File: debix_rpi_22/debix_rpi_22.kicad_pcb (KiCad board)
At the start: 2 copper layers, 71 x 12.5 mm, 2 parts, among them J1 Conn_01x24, J3 RPi 22 Pin MIPI CSI-2

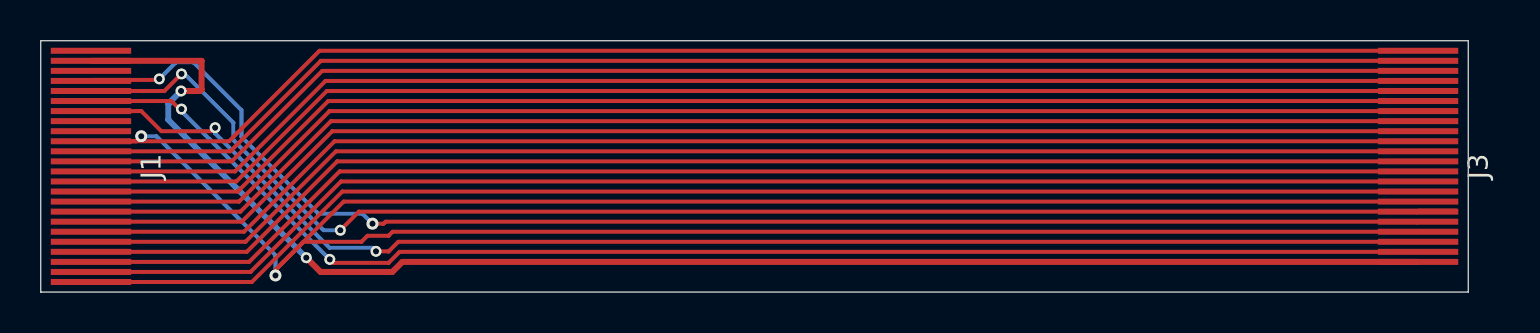
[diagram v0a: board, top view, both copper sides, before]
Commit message: ROUNDED.
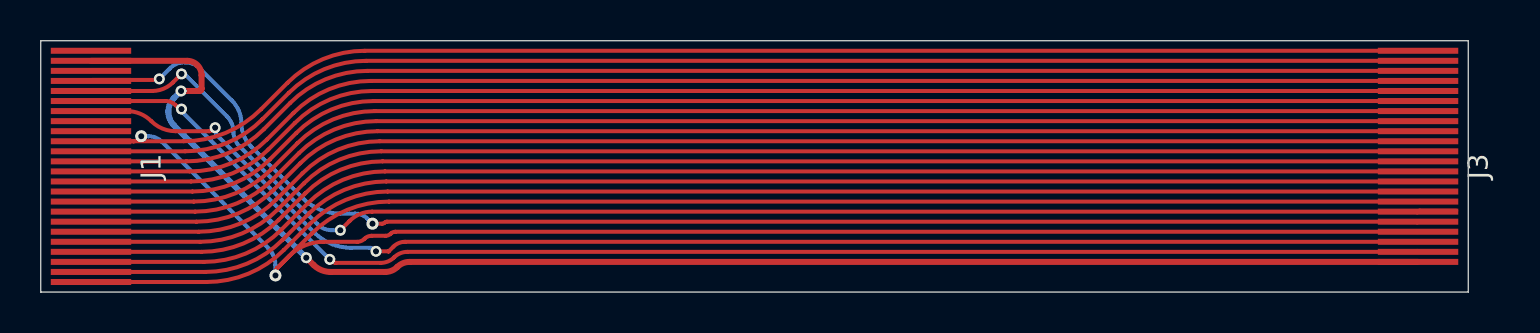
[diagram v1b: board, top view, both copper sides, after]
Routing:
- net GND: track 466.2 -> 463.2 mm
- net +3V3: track 75.2 -> 74.6 mm
- net /csi_d3_P: track 67.9 -> 67.3 mm
- net /csi_d3_N: track 67.9 -> 67.3 mm
- net /csi_d2_P: track 67.9 -> 67.3 mm
- net /csi_clk_N: track 67.9 -> 67.3 mm
- net /csi_d2_N: track 67.9 -> 67.3 mm
- net /csi_d1_P: track 67.9 -> 67.3 mm
- net /csi_d1_N: track 67.9 -> 67.3 mm
- net /csi_d0_P: track 67.9 -> 67.3 mm
- net /csi_d0_N: track 67.9 -> 67.3 mm
- net /csi_clk_P: track 67.9 -> 67.3 mm
